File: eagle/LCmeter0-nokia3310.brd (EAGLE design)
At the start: 160 x 100 mm, 29 parts, among them K1 DS2Y

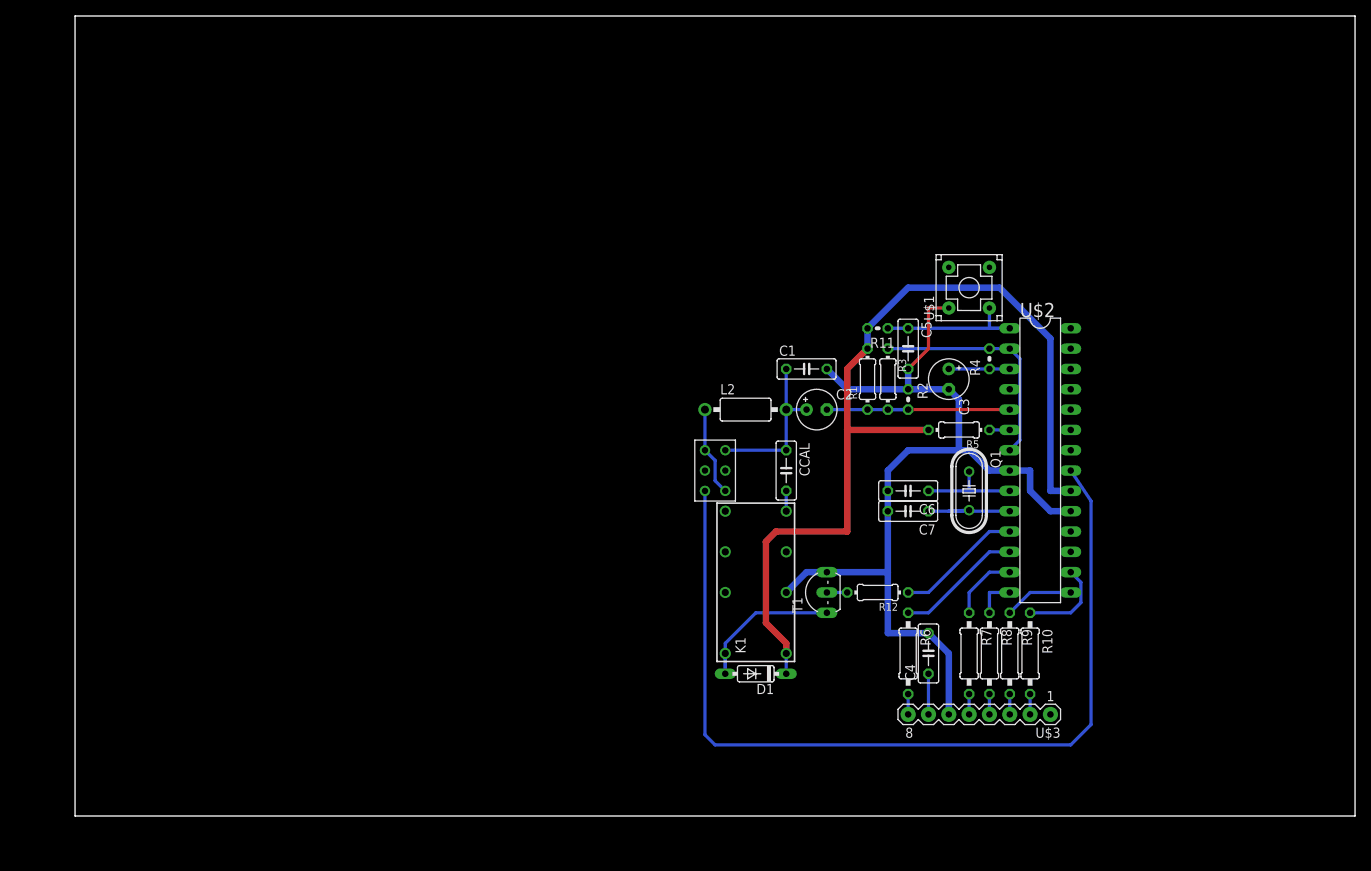
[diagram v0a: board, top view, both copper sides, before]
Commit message: ...
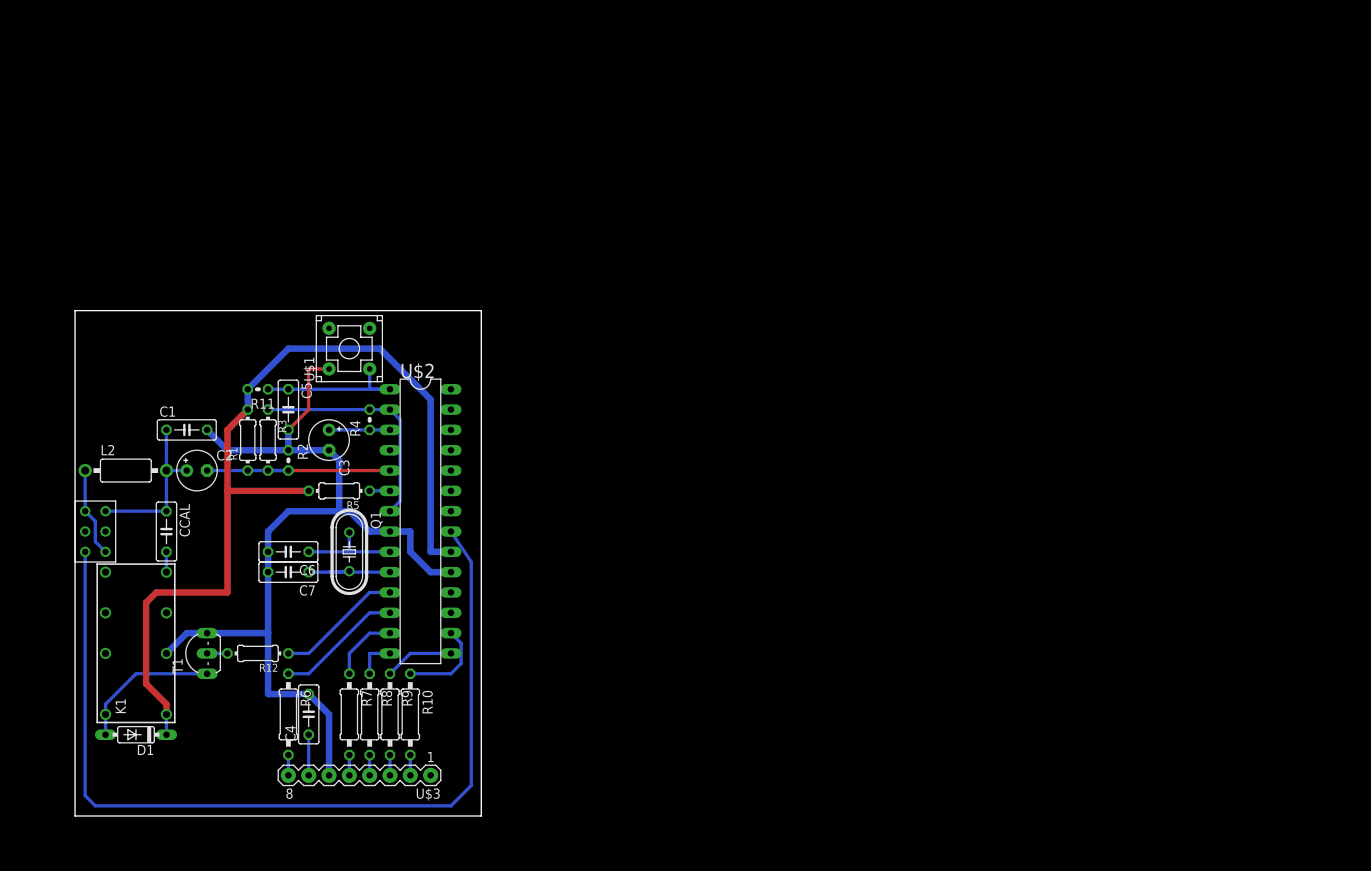
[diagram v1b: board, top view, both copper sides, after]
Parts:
- moved C1 77.8 mm to (14.0, 48.3)
- moved C2 77.8 mm to (15.2, 43.2)
- moved C3 77.8 mm to (31.8, 47.0)
- moved C4 77.8 mm to (29.2, 12.7)
- moved C5 77.8 mm to (26.7, 50.8)
- moved C6 77.8 mm to (26.7, 33.0)
- moved C7 77.8 mm to (26.7, 30.5)
- moved CCAL 77.8 mm to (11.4, 35.6)
- moved D1 77.8 mm to (7.62, 10.2)
- moved K1 77.8 mm to (7.62, 21.6)
- moved L2 77.8 mm to (6.35, 43.2)
- moved Q1 77.8 mm to (34.3, 33.0)
- moved R1 77.8 mm to (21.6, 47.0)
- moved R10 77.8 mm to (41.9, 12.7)
- moved R11 77.8 mm to (22.9, 53.3)
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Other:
- board size 160 x 100 mm -> 50.8 x 63.2 mm

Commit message: ...
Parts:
- U$1: device lc-meter:PB-5 -> mcu:PB-5
- U$2: device lc-meter:DIL28-3 -> mcu:DIL28-3
- U$3: device lc-meter:1X8 -> mcu:1X8
- U$4: device lc-meter:DPDT -> mcu:DPDT
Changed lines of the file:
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@@
 <element name="R9" library="rcl" package="0207/10" value="3.3k" x="39.37" y="12.7" rot="R270"/>
 <element name="T1" library="transistor" package="TO92-CBE" value="" x="16.51" y="20.32" rot="R90"/>
-<element name="U$1" library="lc-meter" package="PB-5" value="PB-SPST" x="34.29" y="58.42" rot="R90"/>
-<element name="U$2" library="lc-meter" package="DIL28-3" value="PIC16F876A-X/SP-COMP" x="43.18" y="36.83" rot="R270"/>
-<element name="U$3" library="lc-meter" package="1X8" value="NOKIA-3310-64X64" x="35.56" y="5.08" rot="R180"/>
-<element name="U$4" library="lc-meter" package="DPDT" value="S-DPDT" x="2.54" y="35.56" rot="R270"/>
+<element name="U$1" library="mcu" package="PB-5" value="PB-SPST" x="34.29" y="58.42" rot="R90"/>
+<element name="U$2" library="mcu" package="DIL28-3" value="PIC16F876A-X/SP-COMP" x="43.18" y="36.83" rot="R270"/>
+<element name="U$3" library="mcu" package="1X8" value="NOKIA-3310-64X64" x="35.56" y="5.08" rot="R180"/>
+<element name="U$4" library="mcu" package="DPDT" value="S-DPDT" x="2.54" y="35.56" rot="R270"/>
 </elements>
 <signals>

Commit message: ...
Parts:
- D1: device diode:DO35-7 -> d:DO35-7
- Q1: device crystal:HC49/S -> q:HC49/S
- T1: device transistor:TO92-CBE -> t:TO92-CBE
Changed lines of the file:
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@@
 <element name="C7" library="rcl" package="C050-025X075" value="22pF" x="26.67" y="30.48" rot="R180"/>
 <element name="CCAL" library="rcl" package="C050-025X075" value="1nF" x="11.43" y="35.56" rot="R270"/>
-<element name="D1" library="diode" package="DO35-7" value="1N4148" x="7.62" y="10.16" rot="R180"/>
+<element name="D1" library="d" package="DO35-7" value="1N4148" x="7.62" y="10.16" rot="R180"/>
 <element name="K1" library="relay" package="DS2Y" value="DS2Y" x="7.62" y="21.59" rot="R90">
 <attribute name="OC_FARNELL" value="unknown" x="7.62" y="21.59" size="1.778" layer="27" rot="R90" display="off"/>
@@
 </element>
 <element name="L2" library="rcl" package="IR-2" value="100uH" x="6.35" y="43.18"/>
-<element name="Q1" library="crystal" package="HC49/S" value="" x="34.29" y="33.02" rot="R270">
+<element name="Q1" library="q" package="HC49/S" value="" x="34.29" y="33.02" rot="R270">
 <attribute name="OC_FARNELL" value="1667008" x="34.29" y="33.02" size="1.778" layer="27" rot="R270" display="off"/>
 <attribute name="OC_NEWARK" value="unknown" x="34.29" y="33.02" size="1.778" layer="27" rot="R270" display="off"/>
@@
 <element name="R8" library="rcl" package="0207/10" value="3.3k" x="36.83" y="12.7" rot="R270"/>
 <element name="R9" library="rcl" package="0207/10" value="3.3k" x="39.37" y="12.7" rot="R270"/>
-<element name="T1" library="transistor" package="TO92-CBE" value="" x="16.51" y="20.32" rot="R90"/>
+<element name="T1" library="t" package="TO92-CBE" value="" x="16.51" y="20.32" rot="R90"/>
 <element name="U$1" library="mcu" package="PB-5" value="PB-SPST" x="34.29" y="58.42" rot="R90"/>
 <element name="U$2" library="mcu" package="DIL28-3" value="PIC16F876A-X/SP-COMP" x="43.18" y="36.83" rot="R270"/>
